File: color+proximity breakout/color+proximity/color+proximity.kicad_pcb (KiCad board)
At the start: 2 copper layers, 31 x 37.6 mm, 34 parts, among them IC1 VL53L4CDV0DH_1, IC2 ISL29125IROZ-T7, J4 Conn_01x05, U6 ICM-20602

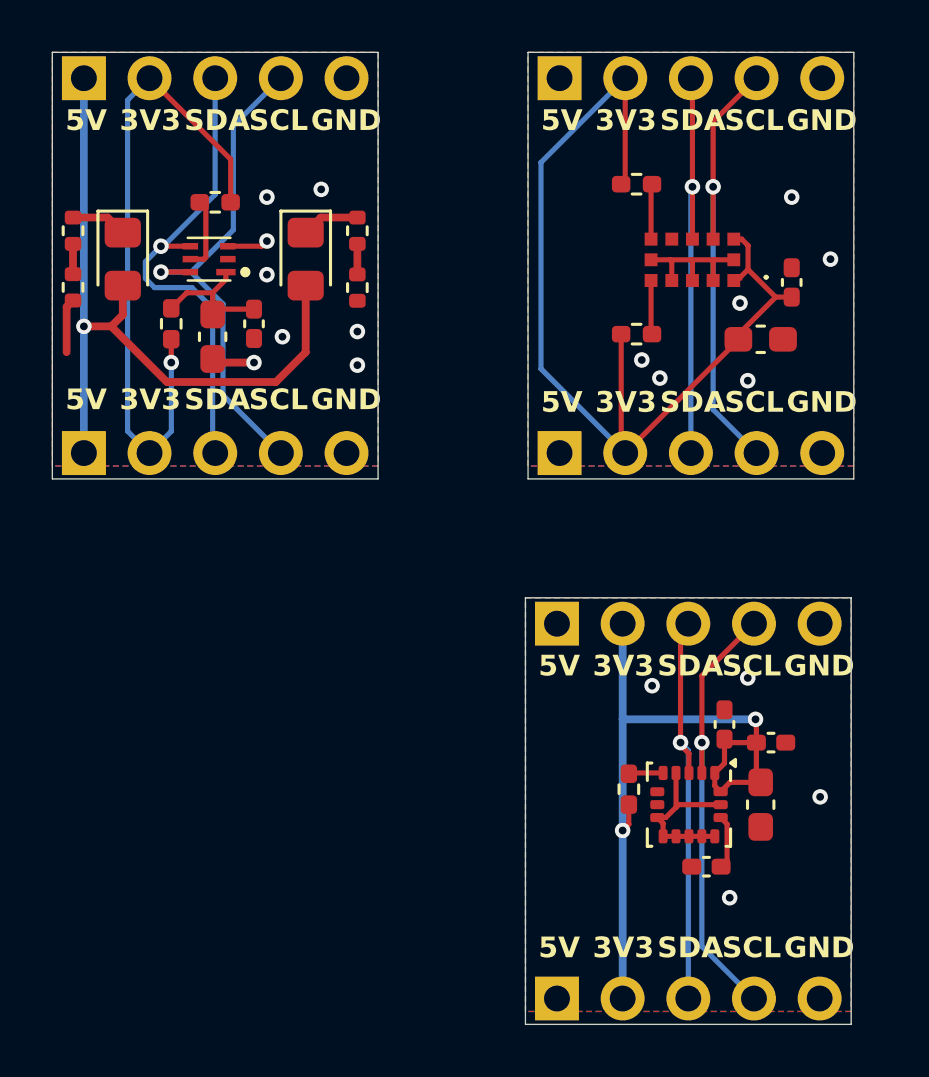
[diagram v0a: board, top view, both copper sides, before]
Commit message: step files and stuff (idk i might have fucked up the settings)
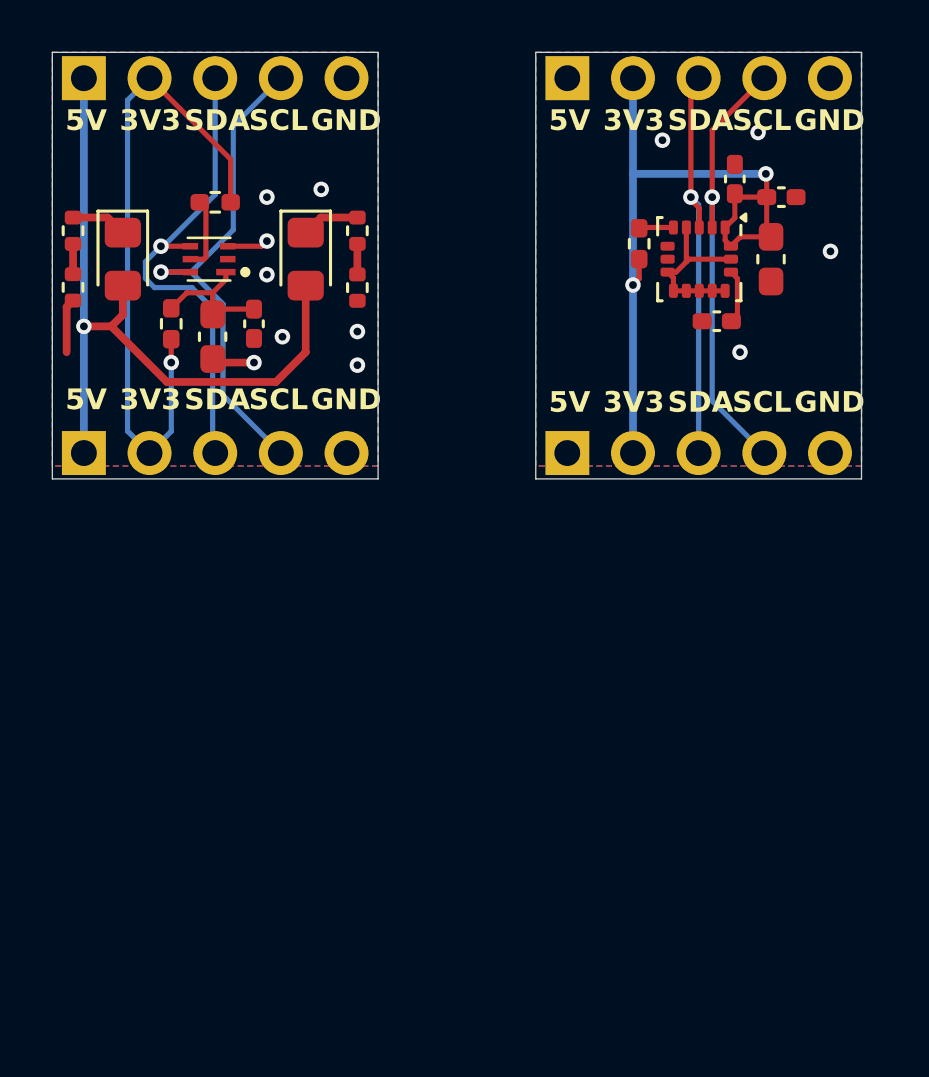
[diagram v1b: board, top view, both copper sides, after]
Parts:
- removed C11: 0.1u, Capacitor_SMD:C_0402_1005Metric_Pad0.74x0.62mm_HandSolder
- removed C12: 4.7u, Capacitor_SMD:C_0603_1608Metric_Pad1.08x0.95mm_HandSolder
- removed the G*** at (124.5, 113.2)
- removed the G*** at (122.9, 108.4)
- removed IC1: VL53L4CDV0DH_1, VL53L4CD:VL53L4CDV0DH1
- removed the J4 at (121.5, 119.6)
- removed the J4 at (121.5, 105.1)
- removed R20, R21: 10k, Resistor_SMD:R_0402_1005Metric_Pad0.72x0.64mm_HandSolder
- moved C9 21.1 mm to (130.1, 109.7)
- moved G*** 21.1 mm to (124.8, 113.2)
- moved J4 21.1 mm to (121.8, 105.1)
- moved C10 21.1 mm to (127.6, 114.5)
- moved C7 21.1 mm to (128.3, 109.0)
- moved C8 21.1 mm to (129.7, 112.1)
- moved G*** 21.1 mm to (123.2, 108.4)
- moved J4 21.1 mm to (121.8, 119.6)
- moved R19 21.1 mm to (124.6, 111.5)
- moved U6 21.1 mm to (126.9, 112.1)
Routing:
- net +3.3V: track 94.2 -> 55.0 mm
- net /scl: track 54.9 -> 37.0 mm, vias 3 -> 2
- net /sda: track 52.0 -> 35.2 mm, vias 3 -> 2
- net GND: track 17.8 -> 12.2 mm, vias 18 -> 12
- net Net-(IC1-GPIO1): track 2.14 -> 0.00 mm
- net Net-(IC1-XSHUT): track 2.09 -> 0.00 mm
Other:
- board size 31 x 37.6 mm -> 31.3 x 16.5 mm
